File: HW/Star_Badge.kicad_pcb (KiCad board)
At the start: 2 copper layers, 180 x 171.6 mm, 55 parts, among them J1 AVR-ISP-6, J2 10118194-0001LF, Q1 Q_NMOS_DGS, Q2 Q_PMOS_DGS, U1 ATTINY861-15XD, U2 TPS613221ADBVT, U3 AP7363-33D-13, X1 Badgelife_sao_connector_v169b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, X2 Badgelife_sao_connector_v169b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, X3 Badgelife_sao_connector_v169b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, X4 Badgelife_sao_connector_v169b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, X5 Badgelife_sao_connector_v169b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

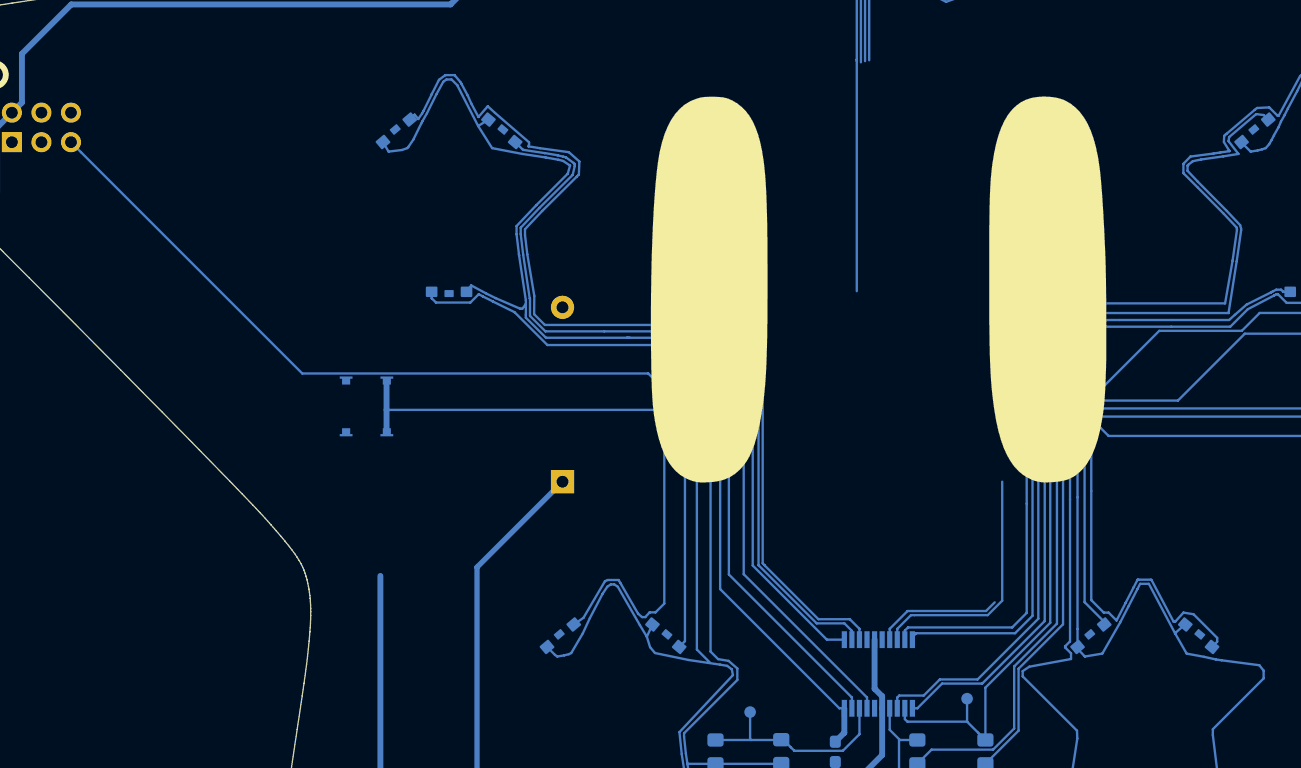
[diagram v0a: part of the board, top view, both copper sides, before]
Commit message: More routing
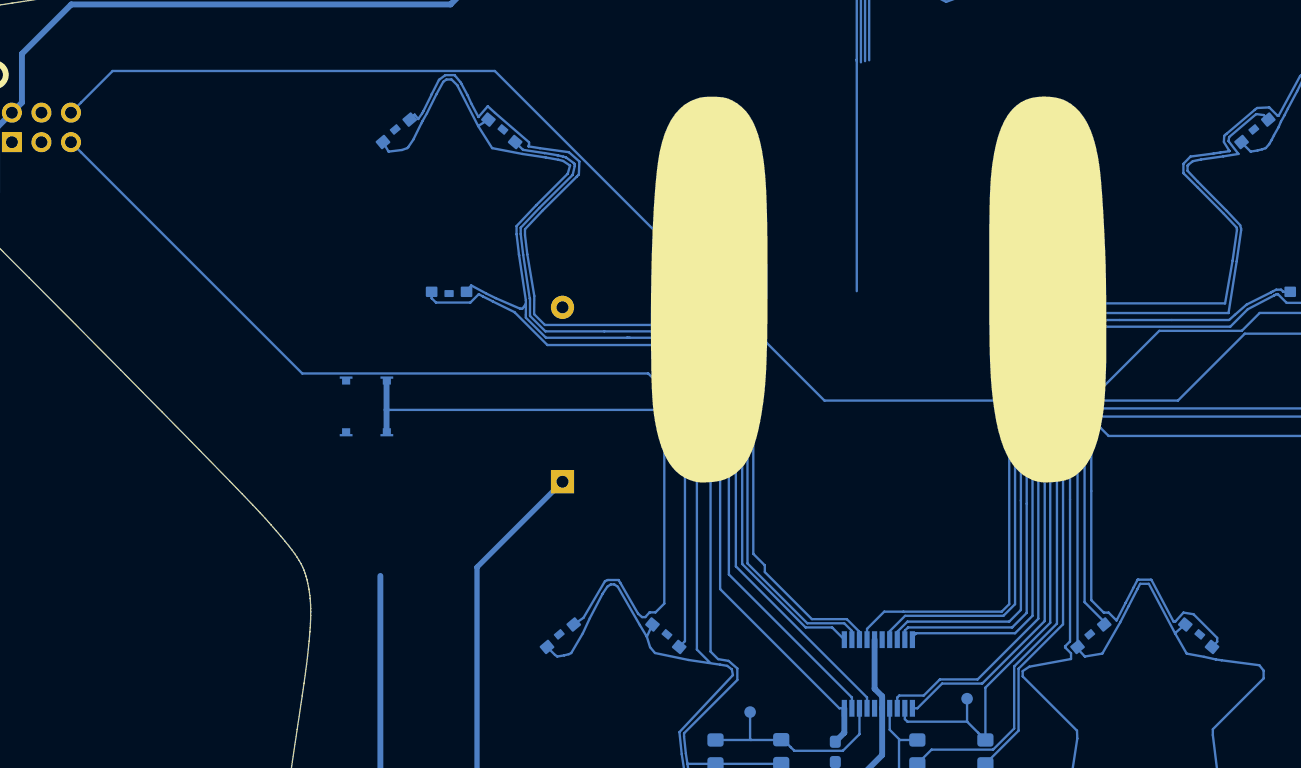
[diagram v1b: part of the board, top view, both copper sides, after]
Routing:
- net /GPIO_2_1: track 21.2 -> 124.9 mm, vias 0 -> 2
- net /EN_RGB1: track 66.3 -> 108.2 mm, vias 0 -> 2
- net /EN_RGB0: track 78.2 -> 103.1 mm, vias 0 -> 2
